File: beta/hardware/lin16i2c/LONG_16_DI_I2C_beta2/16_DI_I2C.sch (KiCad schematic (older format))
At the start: 85 parts, among them P1 CONN_2, P10 CONN_5, P12 CONN_5, P13 CONN_2, P2 CONN_2, P3 CONN_2, P4 CONN_2, P5 CONN_2, P6 CONN_2, P7 CONN_2, P8 CONN_2, U1 PCF8574, U2 PCF8574

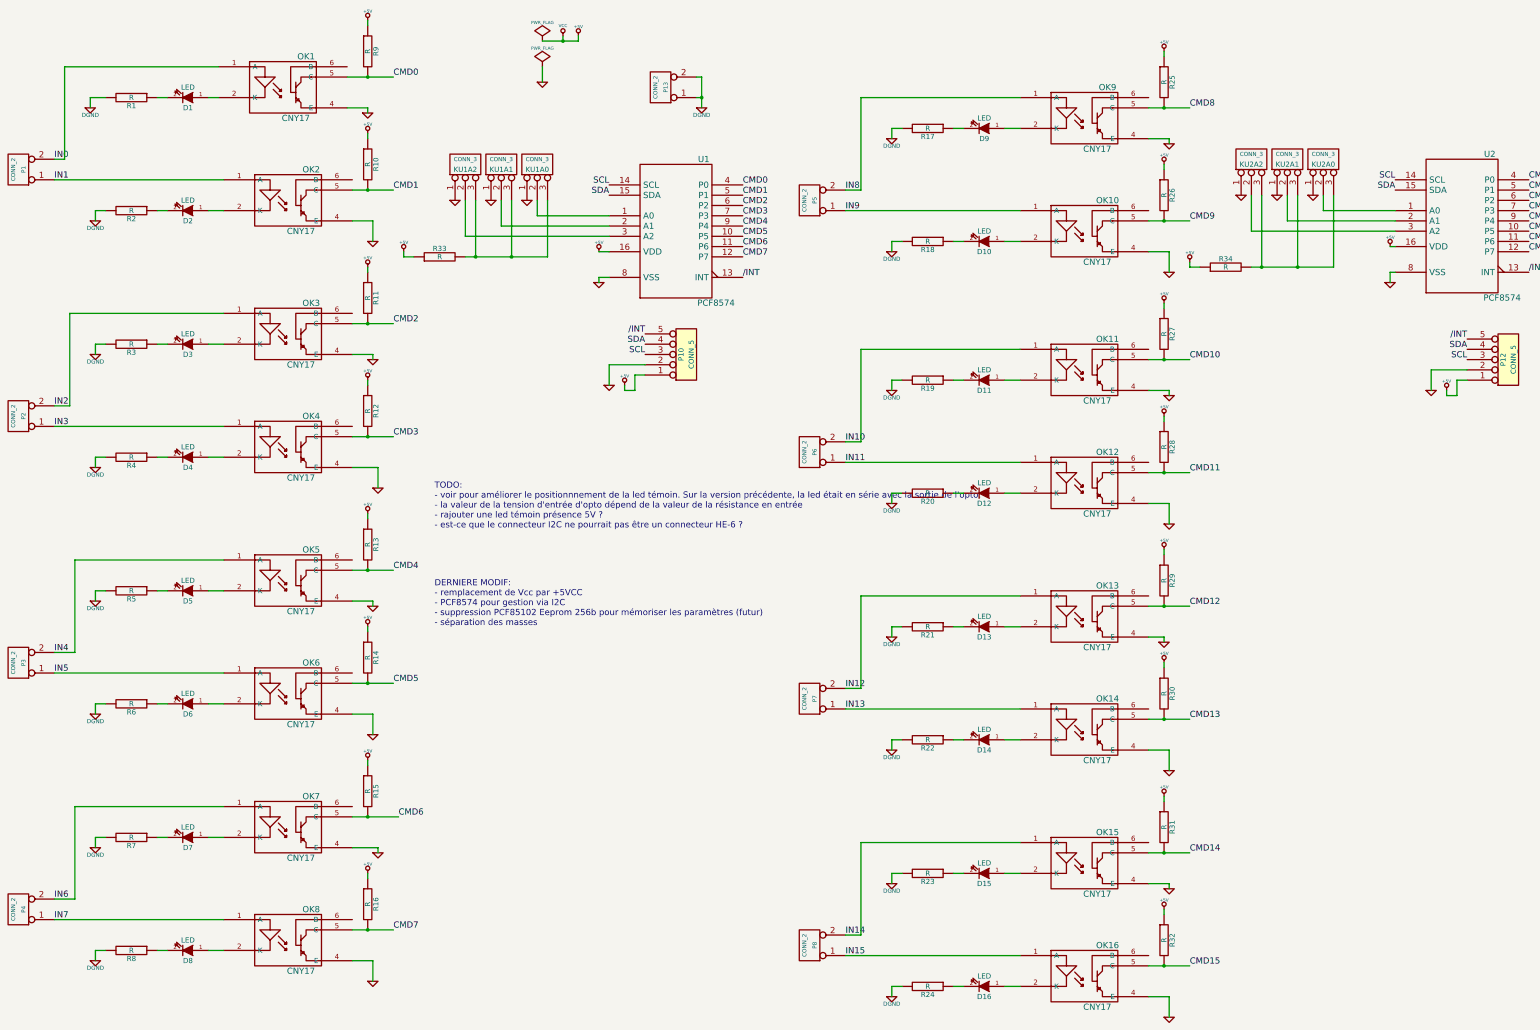
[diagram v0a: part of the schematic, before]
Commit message: routage
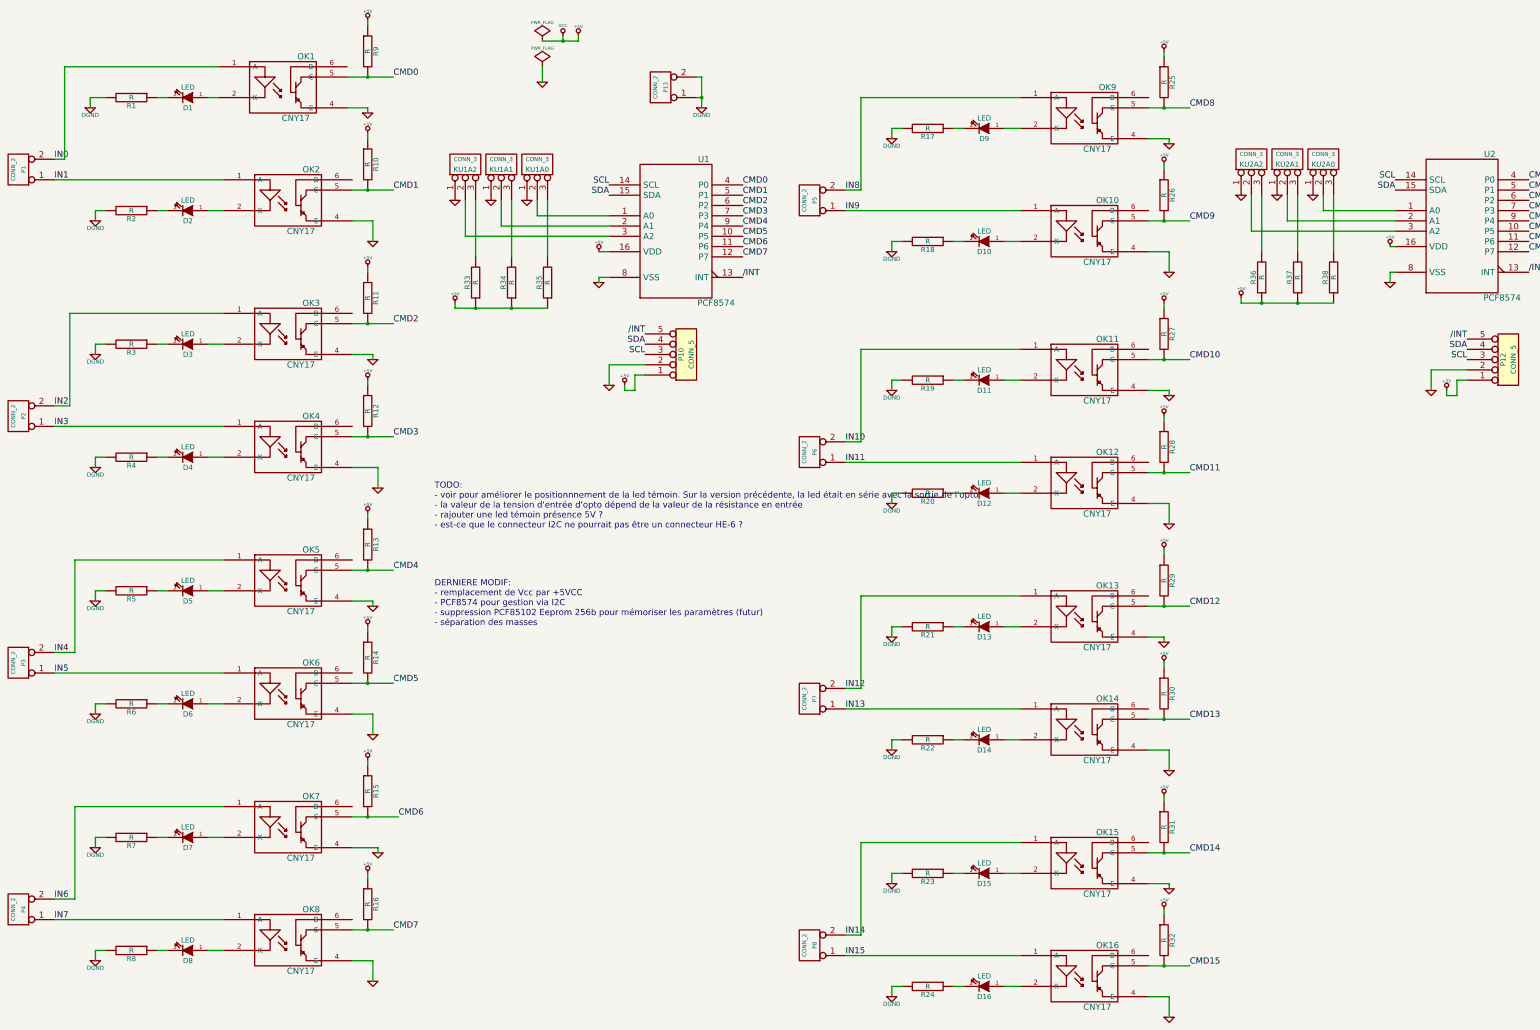
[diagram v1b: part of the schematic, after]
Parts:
- added R35, R36, R37, R38: R, symbol R
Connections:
- net +5V: now also R35.1, R36.1, R37.1, R38.1
- net at KU1A2.3 (P3), R33.2: no longer KU1A0.3 (P3), KU1A1.3 (P3)
- new net: KU1A0.3 (P3), R35.2
- new net: KU1A1.3 (P3), R34.2
- new net: KU2A1.3 (P3), R37.2
- new net: KU2A0.3 (P3), R38.2
- new net: KU2A2.3 (P3), R36.2
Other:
- moved on the sheet: R33
